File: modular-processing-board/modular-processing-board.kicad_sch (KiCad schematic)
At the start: 7 parts

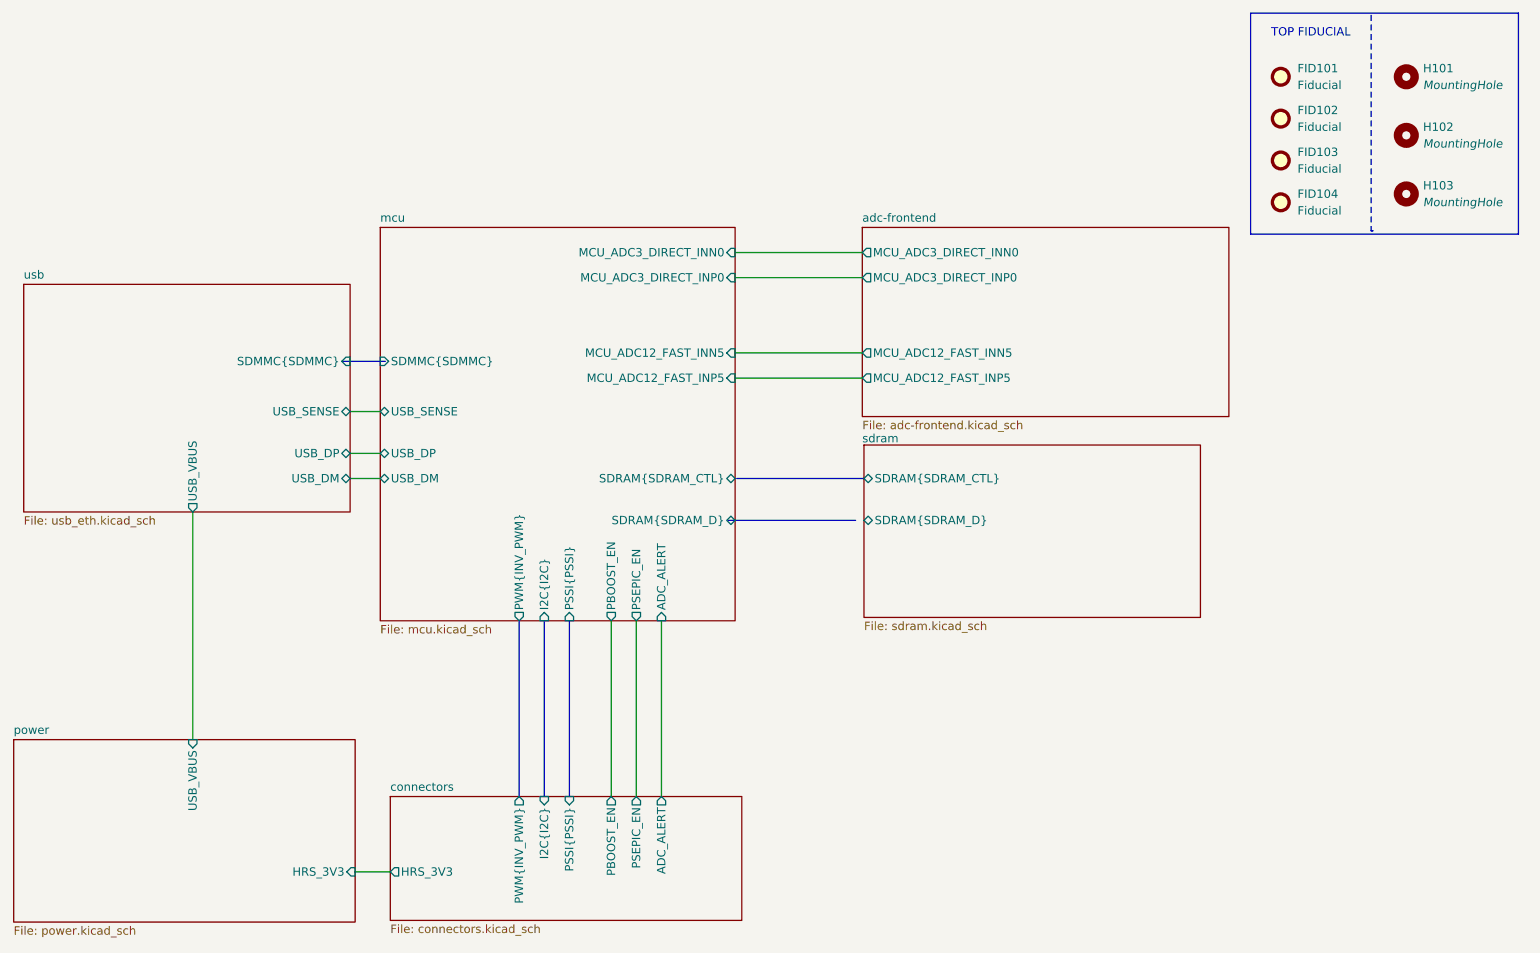
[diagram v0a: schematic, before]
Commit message: completed schematic
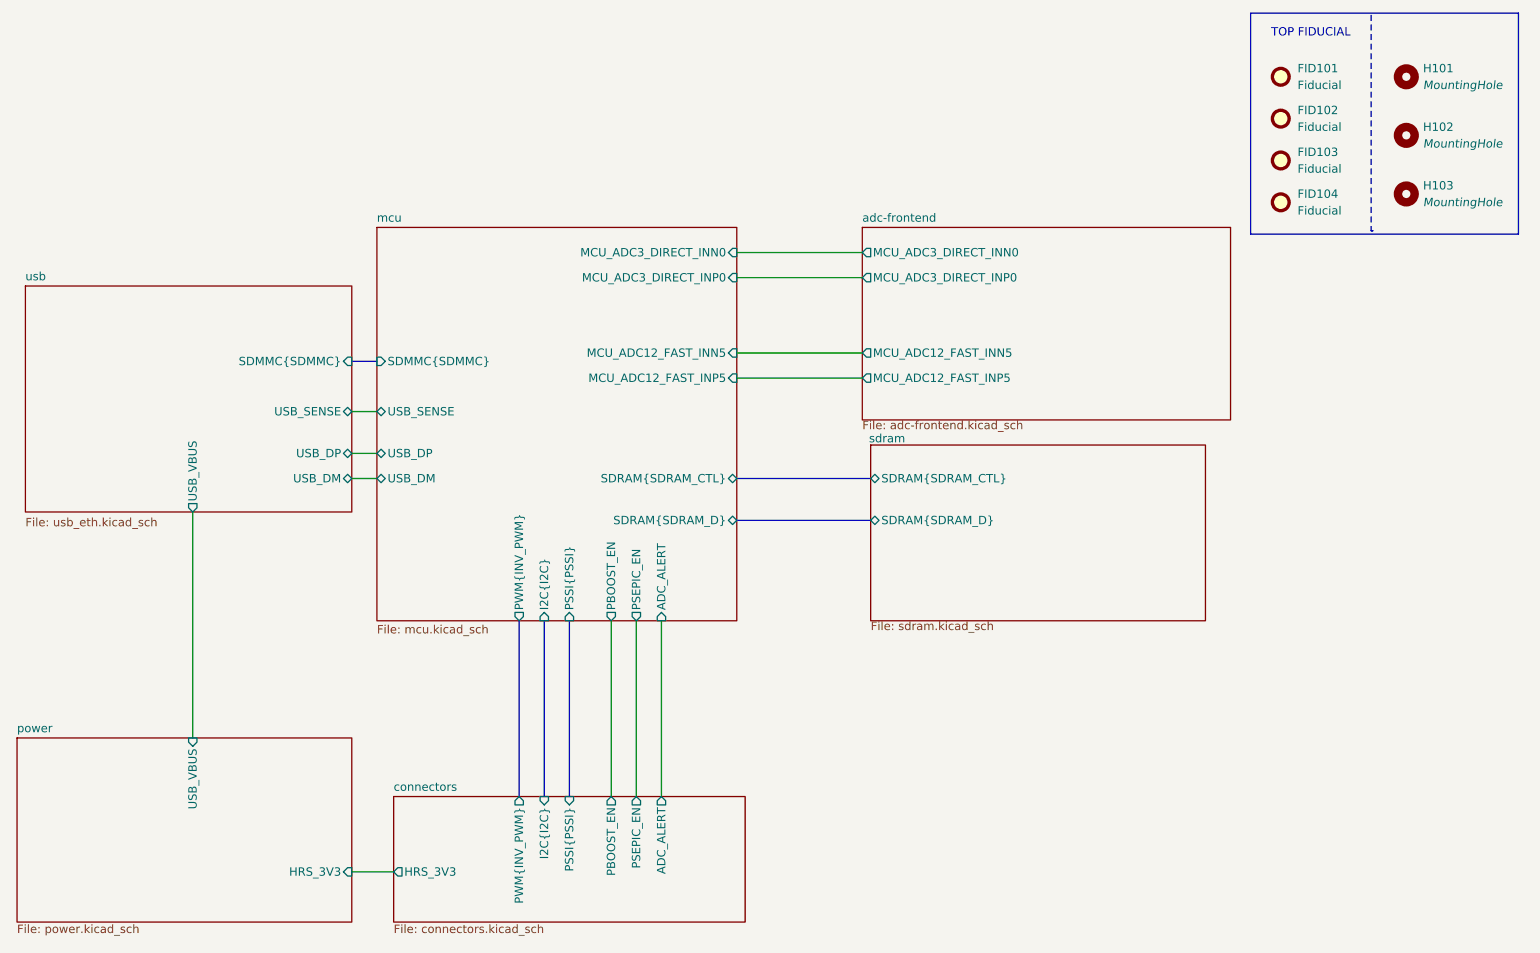
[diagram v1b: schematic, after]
